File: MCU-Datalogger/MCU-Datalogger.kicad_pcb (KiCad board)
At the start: 2 copper layers, 50.8 x 30.5 mm, 29 parts, among them J1 Conn_01x04_Pin, J2 Conn_01x04_Pin, J3 Conn_01x09_Pin, J4 Conn_02x03_Odd_Even, U1 24LC1025, U2 24LC1025, U3 DS1337S+, U4 ATMEGA328P-AU, Y1 32.768 KHz, Y2 16 MHz

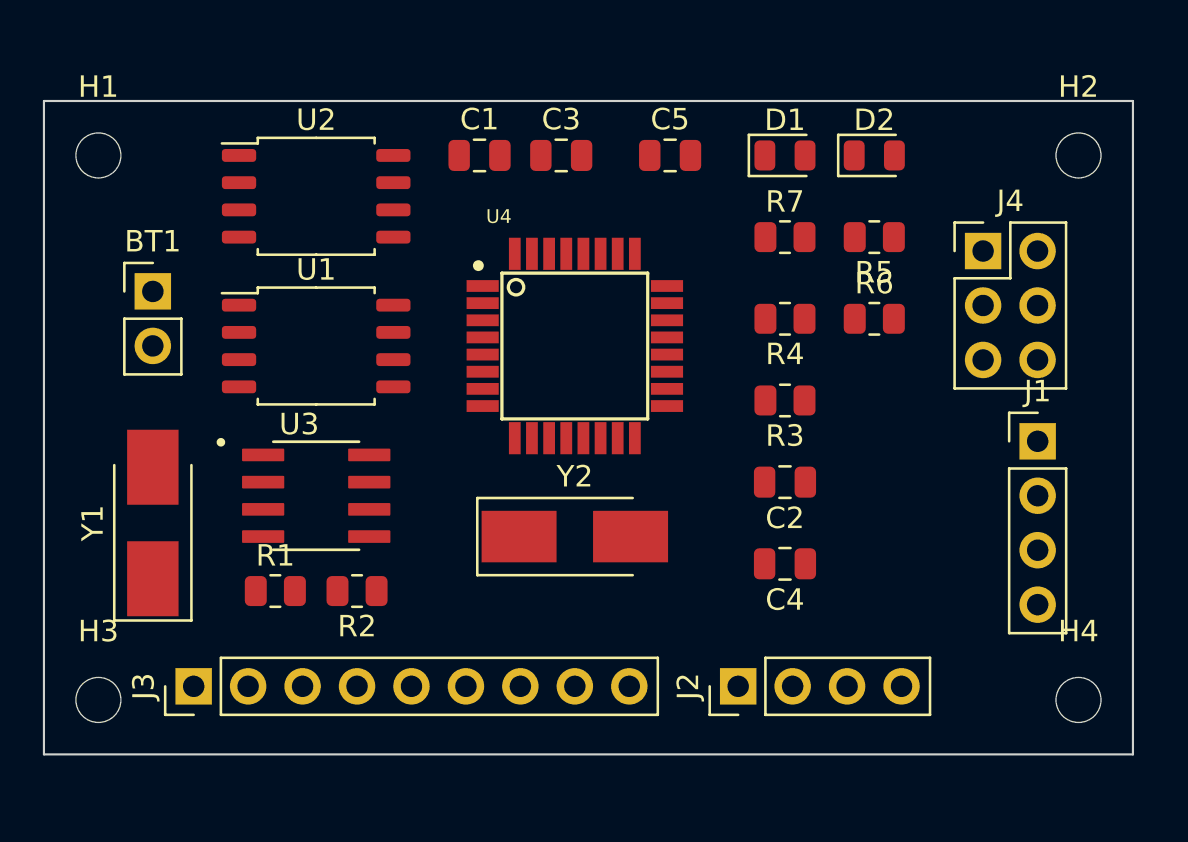
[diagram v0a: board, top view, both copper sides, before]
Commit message: Refine outline
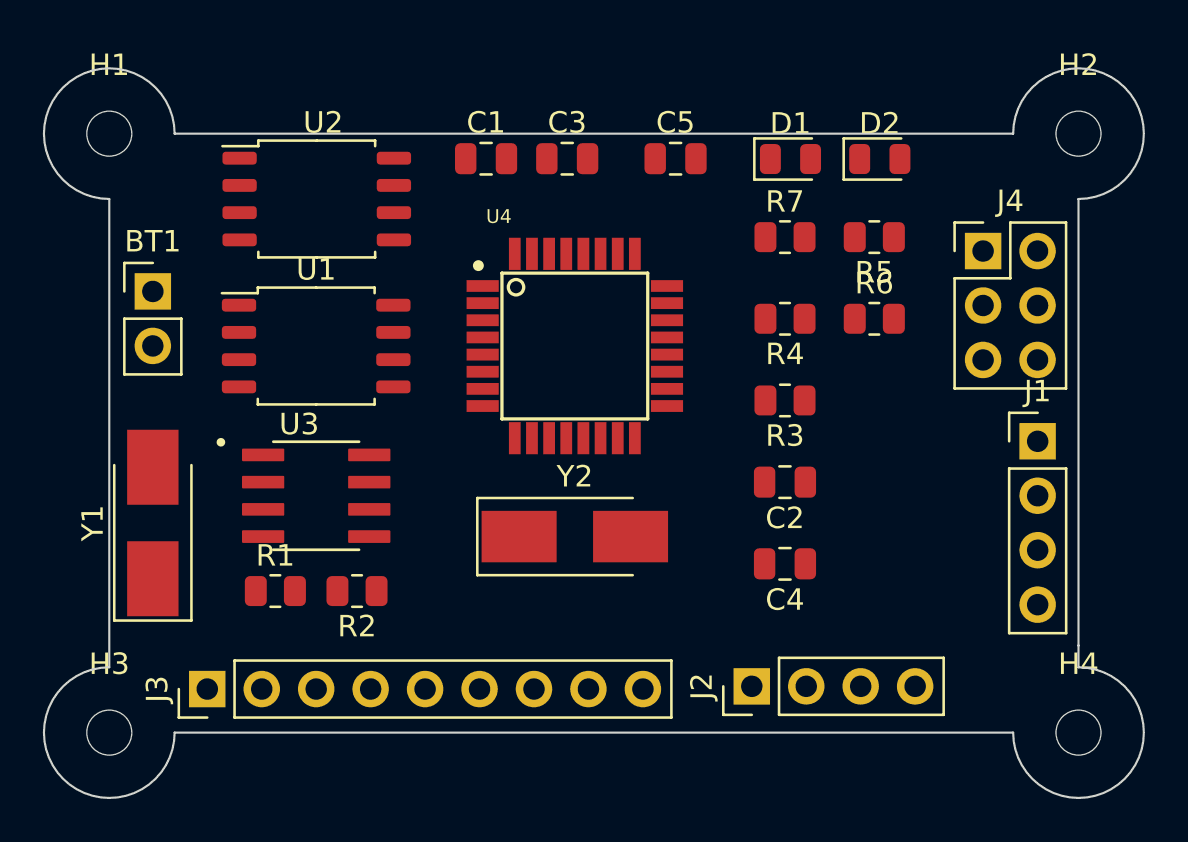
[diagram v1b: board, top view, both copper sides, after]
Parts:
- moved H3 1.61 mm to (130.0, 105.7)
- moved H4 1.52 mm to (175.3, 105.7)
- moved H1 1.14 mm to (130.0, 77.7)
- moved H2 1.02 mm to (175.3, 77.7)
- moved J3 0.65 mm to (134.6, 103.6)
- moved J2 0.64 mm to (160.0, 103.5)
- moved C1 0.34 mm to (147.6, 78.9)
- moved C3 0.32 mm to (151.4, 78.9)
- moved D1 0.31 mm to (161.8, 78.9)
- moved D2 0.31 mm to (166.0, 78.9)
- moved C5 0.30 mm to (156.5, 78.9)
- moved U2 0.13 mm to (139.7, 80.8)
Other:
- board size 50.8 x 30.5 mm -> 51.3 x 34 mm
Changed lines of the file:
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@@
   )
   (footprint "Package_SO:SOIC-8_5.23x5.23mm_P1.27mm" (layer "F.Cu")
-    (at 139.7 80.645)
+    (at 139.7254 80.7724)
     (descr "SOIC, 8 Pin (http://www.winbond.com/resource-files/w25q32jv%20revg%2003272018%20plus.pdf#page=68), generated with kicad-footprint-generator ipc_gullwing_generator.py")
     (tags "SOIC SO")
@@
     (property "ki_keywords" "I2C Serial EEPROM")
     (attr smd)
-    (fp_text reference "U2" (at 0 -3.56) (layer "F.SilkS")
+    (fp_text reference "U2" (at 0.3025 -3.56) (layer "F.SilkS")
         (effects (font (size 1 1) (thickness 0.15)))
     )
@@
   )
   (footprint "Connector_PinHeader_2.54mm:PinHeader_1x04_P2.54mm_Vertical" (layer "F.Cu")
-    (at 159.385 103.505 90)
+    (at 160.02 103.505 90)
     (descr "Through hole straight pin header, 1x04, 2.54mm pitch, single row")
     (tags "Through hole pin header THT 1x04 2.54mm single row")
@@
   )
   (footprint "LED_SMD:LED_0805_2012Metric" (layer "F.Cu")
-    (at 161.5675 78.74)
+    (at 161.8238 78.9074)
     (descr "LED SMD 0805 (2012 Metric), square (rectangular) end terminal, IPC_7351 nominal, (Body size source: https://docs.google.com/spreadsheets/d/1BsfQQcO9C6DZCsRaXUlFlo91Tg2WpOkGARC1WS5S8t0/edit?usp=sharing), generated with kicad-footprint-generator")
     (tags "LED")
@@
   )
   (footprint "Capacitor_SMD:C_0805_2012Metric" (layer "F.Cu")
-    (at 156.21 78.74)
+    (at 156.464 78.8924)
     (descr "Capacitor SMD 0805 (2012 Metric), square (rectangular) end terminal, IPC_7351 nominal, (Body size source: IPC-SM-782 page 76, https://www.pcb-3d.com/wordpress/wp-content/uploads/ipc-sm-782a_amendment_1_and_2.pdf, https://docs.google.com/spreadsheets/d/1BsfQQcO9C6DZCsRaXUlFlo91Tg2WpOkGARC1WS5S8t0/edit?usp=sharing), generated with kicad-footprint-generator")
     (tags "capacitor")
@@
   )
   (footprint "Connector_PinHeader_2.54mm:PinHeader_1x09_P2.54mm_Vertical" (layer "F.Cu")
-    (at 133.985 103.505 90)
+    (at 134.62 103.632 90)
     (descr "Through hole straight pin header, 1x09, 2.54mm pitch, single row")
     (tags "Through hole pin header THT 1x09 2.54mm single row")
@@
   )
   (footprint "MountingHole:MountingHole_2.1mm" (layer "F.Cu")
-    (at 129.54 104.14)
+    (at 130.048 105.664)
     (descr "Mounting Hole 2.1mm, no annular")
     (tags "mounting hole 2.1mm no annular")
@@
   )
   (footprint "LED_SMD:LED_0805_2012Metric" (layer "F.Cu")
-    (at 165.735 78.74)
+    (at 165.9913 78.9074)
     (descr "LED SMD 0805 (2012 Metric), square (rectangular) end terminal, IPC_7351 nominal, (Body size source: https://docs.google.com/spreadsheets/d/1BsfQQcO9C6DZCsRaXUlFlo91Tg2WpOkGARC1WS5S8t0/edit?usp=sharing), generated with kicad-footprint-generator")
     (tags "LED")
@@
   )
   (footprint "MountingHole:MountingHole_2.1mm" (layer "F.Cu")
-    (at 175.26 104.14)
+    (at 175.26 105.664)
     (descr "Mounting Hole 2.1mm, no annular")
     (tags "mounting hole 2.1mm no annular")
@@
   )
   (footprint "Capacitor_SMD:C_0805_2012Metric" (layer "F.Cu")
-    (at 147.32 78.74)
+    (at 147.6248 78.8924)
     (descr "Capacitor SMD 0805 (2012 Metric), square (rectangular) end terminal, IPC_7351 nominal, (Body size source: IPC-SM-782 page 76, https://www.pcb-3d.com/wordpress/wp-content/uploads/ipc-sm-782a_amendment_1_and_2.pdf, https://docs.google.com/spreadsheets/d/1BsfQQcO9C6DZCsRaXUlFlo91Tg2WpOkGARC1WS5S8t0/edit?usp=sharing), generated with kicad-footprint-generator")
     (tags "capacitor")
@@
   )
   (footprint "MountingHole:MountingHole_2.1mm" (layer "F.Cu")
-    (at 129.54 78.74)
+    (at 130.048 77.724)
     (descr "Mounting Hole 2.1mm, no annular")
     (tags "mounting hole 2.1mm no annular")
@@
   )
   (footprint "MountingHole:MountingHole_2.1mm" (layer "F.Cu")
-    (at 175.26 78.74)
+    (at 175.26 77.724)
     (descr "Mounting Hole 2.1mm, no annular")
     (tags "mounting hole 2.1mm no annular")
@@
   )
   (footprint "Capacitor_SMD:C_0805_2012Metric" (layer "F.Cu")
-    (at 151.13 78.74)
+    (at 151.4094 78.8924)
     (descr "Capacitor SMD 0805 (2012 Metric), square (rectangular) end terminal, IPC_7351 nominal, (Body size source: IPC-SM-782 page 76, https://www.pcb-3d.com/wordpress/wp-content/uploads/ipc-sm-782a_amendment_1_and_2.pdf, https://docs.google.com/spreadsheets/d/1BsfQQcO9C6DZCsRaXUlFlo91Tg2WpOkGARC1WS5S8t0/edit?usp=sharing), generated with kicad-footprint-generator")
     (tags "capacitor")
@@
     )
   )
-  (gr_rect (start 127 76.2) (end 177.8 106.68)
-    (stroke (width 0.1) (type default)) (fill none) (layer "Edge.Cuts"))
+  (gr_line (start 133.096 105.664) (end 172.212 105.664)
+    (stroke (width 0.1) (type default)) (layer "Edge.Cuts"))
+  (gr_line (start 175.26 101.6) (end 175.26 80.772)
+    (stroke (width 0.1) (type default)) (layer "Edge.Cuts"))
+  (gr_line (start 130.048 80.772) (end 130.048 102.616)
+    (stroke (width 0.1) (type default)) (layer "Edge.Cuts"))
+  (gr_arc (start 130.048 80.772) (mid 127.892739 75.568739) (end 133.096 77.724)
+    (stroke (width 0.1) (type default)) (layer "Edge.Cuts"))
+  (gr_line (start 172.212 77.724) (end 133.096 77.724)
+    (stroke (width 0.1) (type default)) (layer "Edge.Cuts"))
+  (gr_arc (start 172.212 77.724) (mid 177.415261 75.568739) (end 175.26 80.772)
+    (stroke (width 0.1) (type default)) (layer "Edge.Cuts"))
+  (gr_arc (start 133.096 105.664) (mid 127.892739 107.819261) (end 130.048 102.616)
+    (stroke (width 0.1) (type default)) (layer "Edge.Cuts"))
+  (gr_line (start 175.26 102.616) (end 175.26 101.6)
+    (stroke (width 0.1) (type default)) (layer "Edge.Cuts"))
+  (gr_arc (start 175.26 102.616) (mid 177.415261 107.819261) (end 172.212 105.664)
+    (stroke (width 0.1) (type default)) (layer "Edge.Cuts"))
 )
